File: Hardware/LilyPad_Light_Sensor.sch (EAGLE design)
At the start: 9 parts, among them U1 TEMT6000

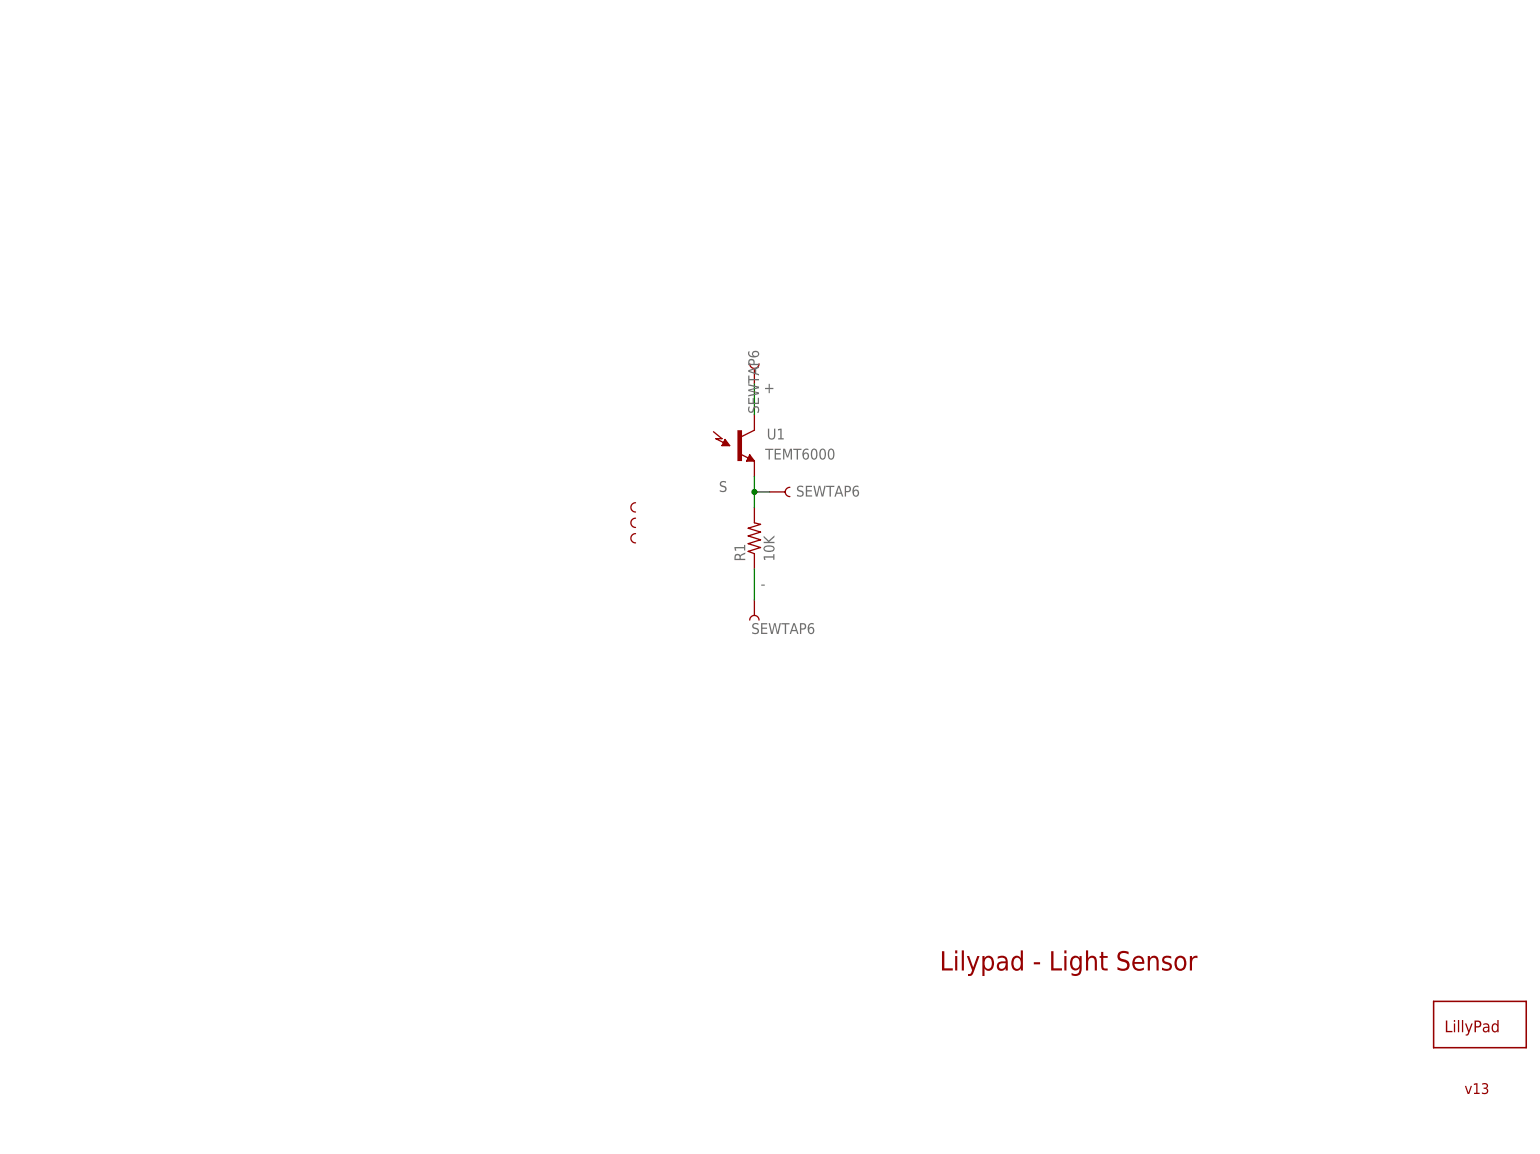
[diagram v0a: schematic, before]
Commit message: Initial Commit
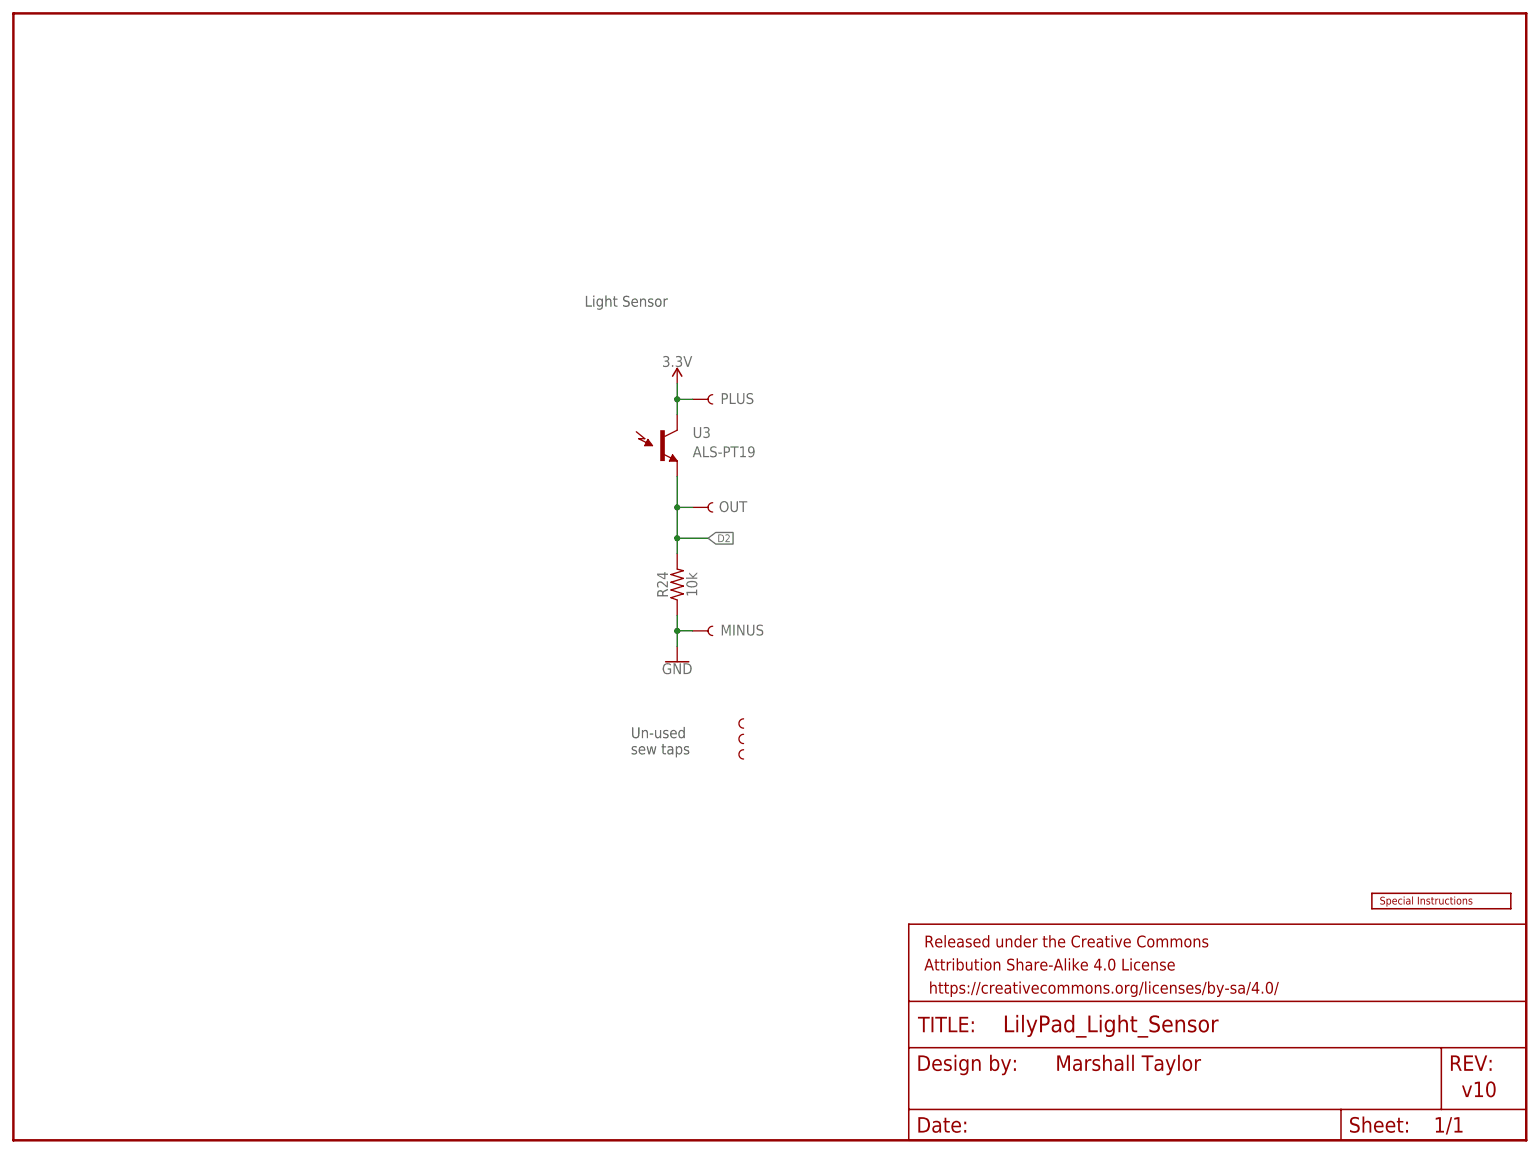
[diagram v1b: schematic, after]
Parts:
- removed LIGHT+, LIGHT-, LIGHTS: SEWTAP6, LilyPad-Wearables:SEWTAP6
- removed LIGHT1, LIGHT2, LIGHT3: SEWTAP-NOHOLE2, LilyPad-Wearables:SEWTAP-NOHOLE2
- removed R1: 10K, SparkFun:RESISTOR0402
- removed U$2: LOGO-LPLP, LilyPad-Wearables:LOGO-LPLP
- removed U1: TEMT6000, SparkFun:TEMT6000
- added FRAME2: FRAME-LETTER, SparkFun-Aesthetics:FRAME-LETTER
- added R24: 10k, SparkFun-Resistors:10KOHM-0603-1/10W-1%
- added SEWTAPLS+: PLUS, LilyPad-Wearables:SEWTAP_SMALL-2SIDE
- added SEWTAPLS-: MINUS, LilyPad-Wearables:SEWTAP_SMALL-2SIDE
- added SEWTAPLSOUT: OUT, LilyPad-Wearables:SEWTAP_SMALL-2SIDE
- added ST1, ST2, ST3: SEWTAP-NOHOLE_SM_NH, LilyPad-Wearables:SEWTAP-NOHOLE_SM_NH
- added U$1: SPECIAL_INSTRUCTIONS-ORDERING, SparkFun-Aesthetics:SPECIAL_INSTRUCTIONS-ORDERING
- added U3: ALS-PT19, SparkFun-Sensors:LIGHT_SENSORALS
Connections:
- removed net +: LIGHT+.1, U1.C1
- removed net -: LIGHT-.1, R1.1
- removed net S: LIGHTS.1, R1.2, U1.E1
- new net 3.3V: SEWTAPLS+.1, U3.C1
- new net D2: R24.2, SEWTAPLSOUT.1, U3.E1
- new net GND: R24.1, SEWTAPLS-.1
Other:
- note added: "Light Sensor"
- note added: "Marshall Taylor"
- note added: "Un-used sew taps"
- note added: "v10"
- note removed: "Lilypad - Light Sensor"
- note removed: "v13"
